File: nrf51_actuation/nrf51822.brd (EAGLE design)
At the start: 58 x 58 mm, 40 parts, among them T1 MMUN2238

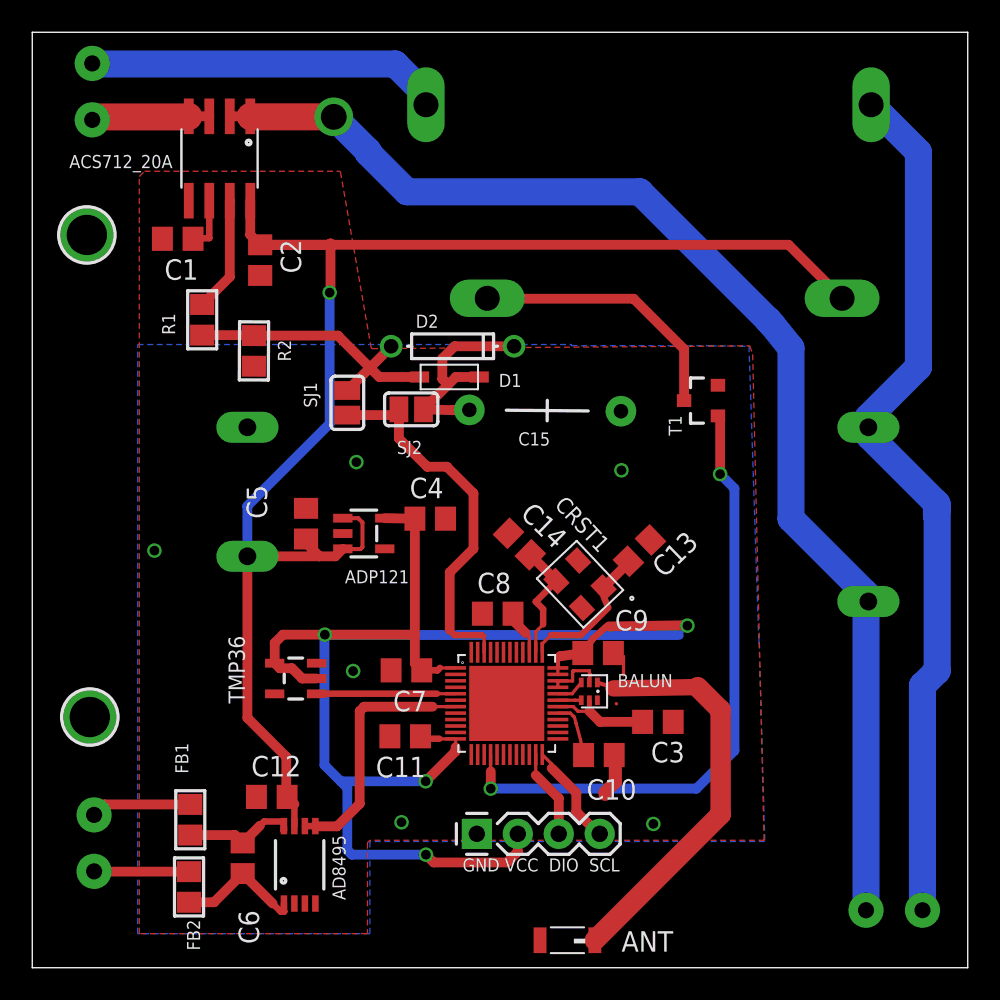
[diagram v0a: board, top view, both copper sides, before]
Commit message: Sent to smart-prototype Actuation 1.2 Compact 1.1
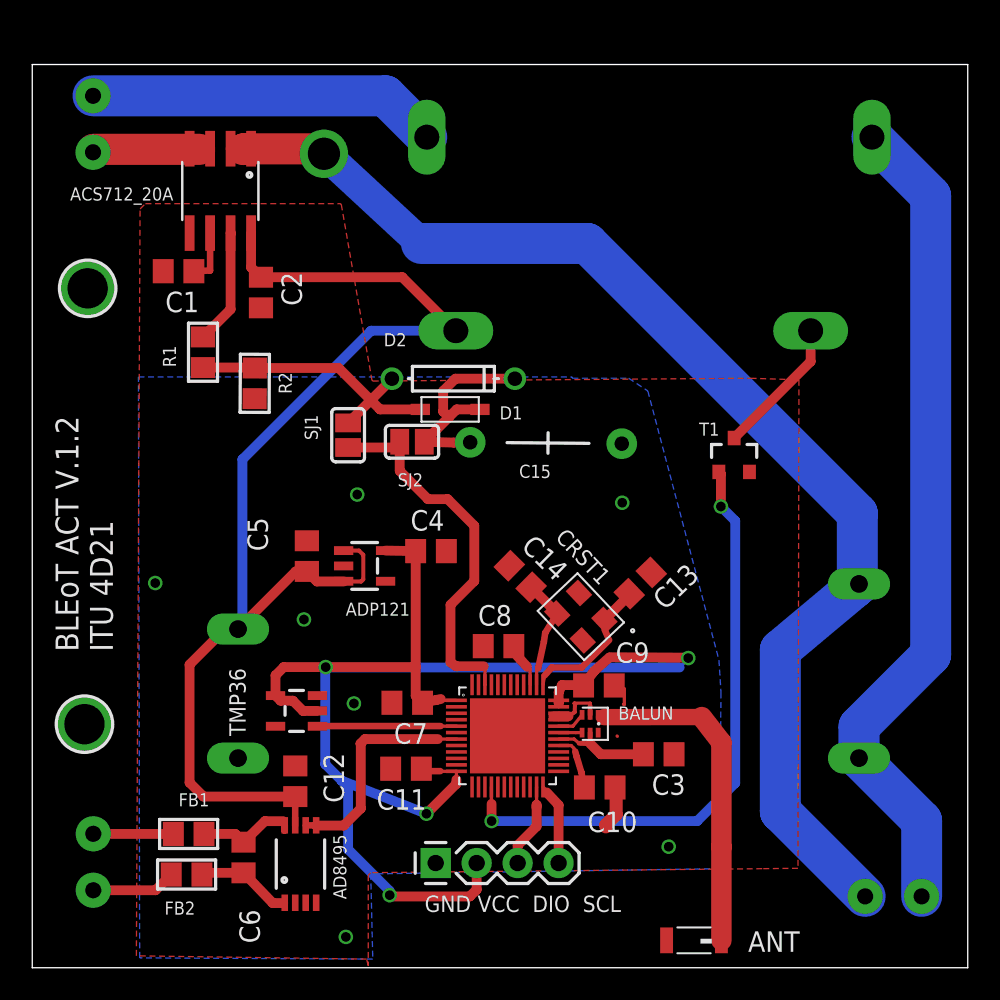
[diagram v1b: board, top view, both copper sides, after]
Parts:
- moved ANT 7.85 mm to (41.0, 1.70)
- moved T1 3.97 mm to (43.5, 31.7), turned to 0 degrees
- moved U$7 3.31 mm to (3.44, 42.1)
- moved JP1 3.13 mm to (25.0, 6.49)
- moved ACS712_20A 2.01 mm to (11.7, 48.2)
- moved C1 2.01 mm to (9.07, 43.2)
- moved D1 2.01 mm to (25.9, 34.6)
- moved SJ1 2.01 mm to (19.6, 33.0)
- moved FTR-K3AB 2.01 mm to (38.3, 45.2), flipped to the top
- moved ADP121 2.01 mm to (20.6, 24.9)
- moved C10 2.01 mm to (35.2, 11.2)
- moved C14 2.01 mm to (30.3, 24.3)
- moved C5 2.01 mm to (17.0, 25.5)
- moved TMP36 2.01 mm to (16.4, 15.9)
- moved C7 2.01 mm to (23.2, 16.4)
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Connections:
- net AC/L: now also FTR-K3AB.3; no longer FTR-K3AB.4
- net AC/LOUT: now also FTR-K3AB.4; no longer FTR-K3AB.3
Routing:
- net 5.0V: track 96.0 -> 76.0 mm, vias 1 -> 0
- net N$7: track 16.7 -> 8.62 mm
- net VDD: track 101.6 -> 97.5 mm
- net N$3: track 25.8 -> 21.7 mm
- net AC/L: track 55.9 -> 52.0 mm
- net N$16: track 8.12 -> 5.98 mm
- net GIOP2: track 39.4 -> 37.9 mm
- net AIN4: track 15.8 -> 14.5 mm
- net N$8: track 6.23 -> 4.97 mm
- net AC/NOUT: track 7.45 -> 8.68 mm
- net GND: track 8.84 -> 9.95 mm, vias 6 -> 7
- net N$9: track 7.44 -> 6.59 mm
- net N$17: track 5.92 -> 5.24 mm
- net N$14: track 6.44 -> 5.93 mm
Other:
- board size 58 x 58 mm -> 58 x 56 mm
- board text added: "BLEoT ACT V.1.2 ITU 4D21"
